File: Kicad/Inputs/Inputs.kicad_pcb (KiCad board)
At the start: 2 copper layers, 7 parts, among them J1 5V, J2 GROUND, J3 Conn_01x05_Female, J4 ACC OUT

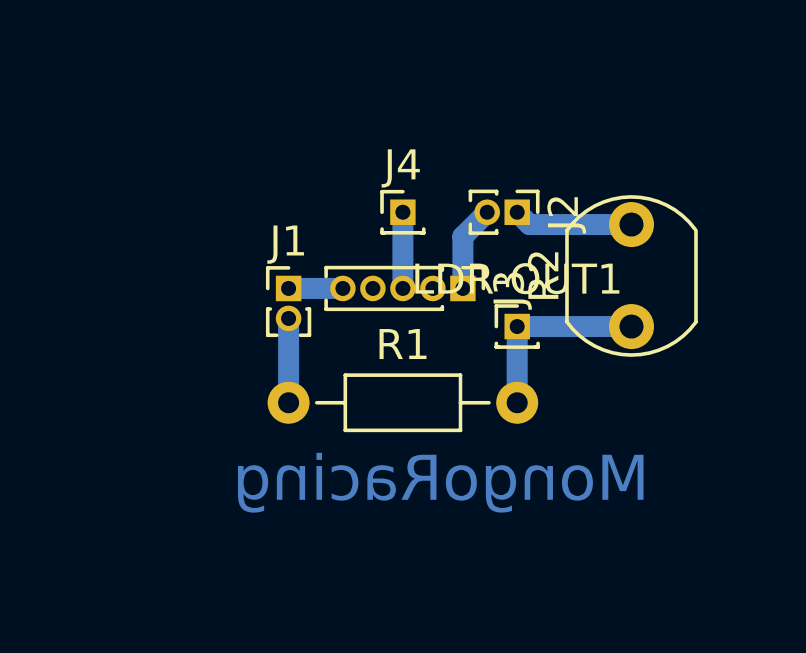
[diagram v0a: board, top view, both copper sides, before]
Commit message: h
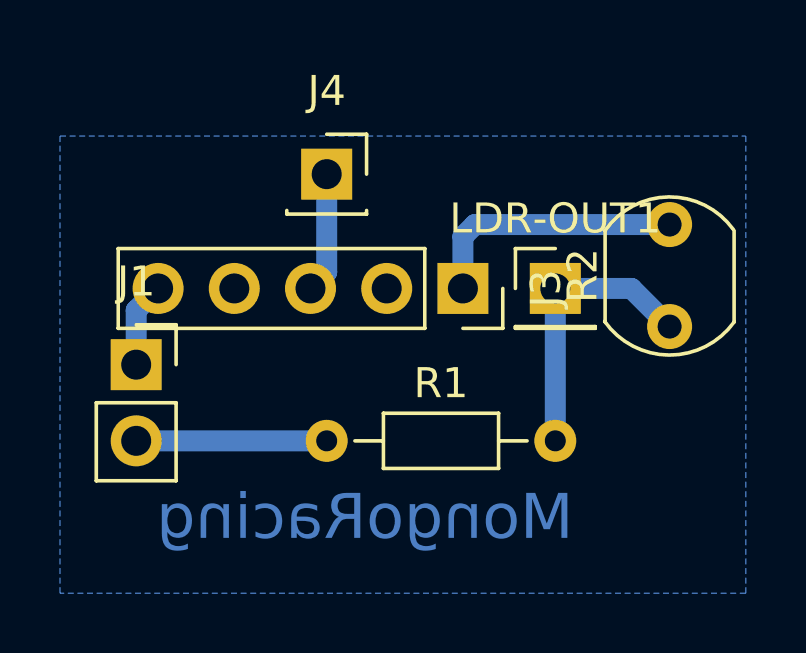
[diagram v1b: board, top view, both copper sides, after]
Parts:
- removed J2: GROUND, Connector_PinHeader_1.00mm:PinHeader_1x02_P1.00mm_Vertical
- J1: footprint Connector_PinHeader_1.00mm:PinHeader_1x02_P1.00mm_Vertical -> Connector_PinSocket_2.54mm:PinSocket_1x02_P2.54mm_Vertical
- J3: footprint Connector_PinHeader_1.00mm:PinHeader_1x05_P1.00mm_Vertical -> Connector_PinSocket_2.54mm:PinSocket_1x05_P2.54mm_Vertical
- J4: footprint Connector_PinHeader_1.00mm:PinHeader_1x01_P1.00mm_Vertical -> Connector_PinSocket_2.54mm:PinSocket_1x01_P2.54mm_Vertical
- LDR-OUT1: footprint Connector_PinHeader_1.00mm:PinHeader_1x01_P1.00mm_Vertical -> Connector_PinHeader_2.54mm:PinHeader_1x01_P2.54mm_Vertical
- moved J1 5.68 mm to (129.5, 85.1)
- moved J4 2.84 mm to (135.9, 78.7)
- moved LDR-OUT1 1.80 mm to (143.5, 82.5)
- moved R1 1.80 mm to (135.9, 87.6)
- moved R2 1.27 mm to (147.3, 83.8)
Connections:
- J3 pad 1: Net-(J2-Pad2) -> Earth
- R2 pad 2: Net-(J2-Pad1) -> Earth
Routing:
- net Earth: track 0.00 -> 8.79 mm
- net Net-(J2-Pad1): track 3.98 -> 0.00 mm
- net Net-(J1-Pad2): track 2.81 -> 6.35 mm
- net Net-(LDR-OUT1-Pad1): track 6.35 -> 9.42 mm
- net Net-(J2-Pad2): track 2.88 -> 0.00 mm
- net Net-(J3-Pad3): track 2.54 -> 4.03 mm
- net Net-(J1-Pad1): track 1.81 -> 2.84 mm
- added copper zone on B.Cu, net Earth
